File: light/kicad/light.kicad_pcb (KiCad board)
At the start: 4 copper layers, 24 x 55.9 mm, 103 parts, among them J1 Conn_01x03_Pin, J2 Conn_01x02_Pin, J3 SPI Socket, U1 FT4232H, U11 TLV7103318DDSE, U14 74LVC1G07, U2 SN74AVC4T774RSVR, U3 SN74AVC4T774RSVR, U4 SN74AVC4T774RSVR, U5 74LVC1G07, U6 SN74AHC595QWBQBRQ1, U7 TLV75533PDBV, U8 TLV75533PDBV, U9 93LC56BT-I/OT, Y1 12MHz_7M-12.000MAAJ

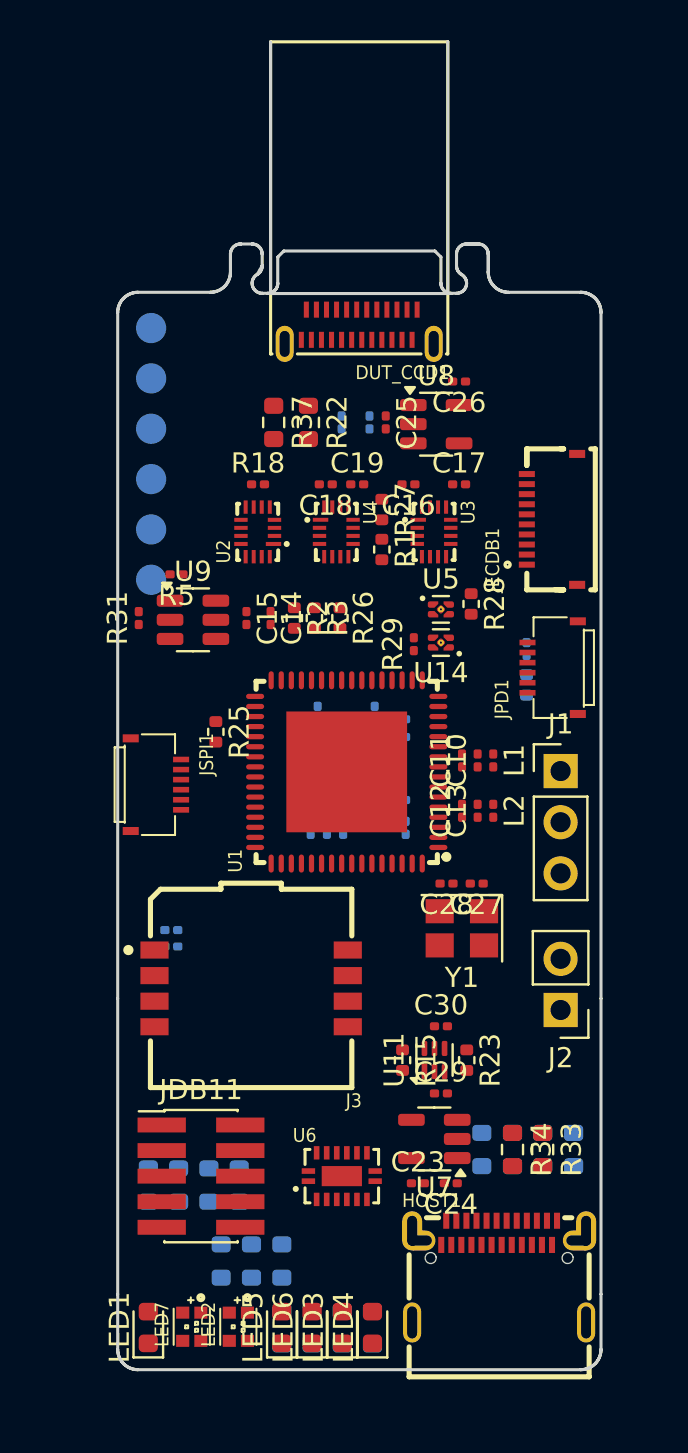
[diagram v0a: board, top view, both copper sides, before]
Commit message: kicad: Update board file layout routing
update board file.
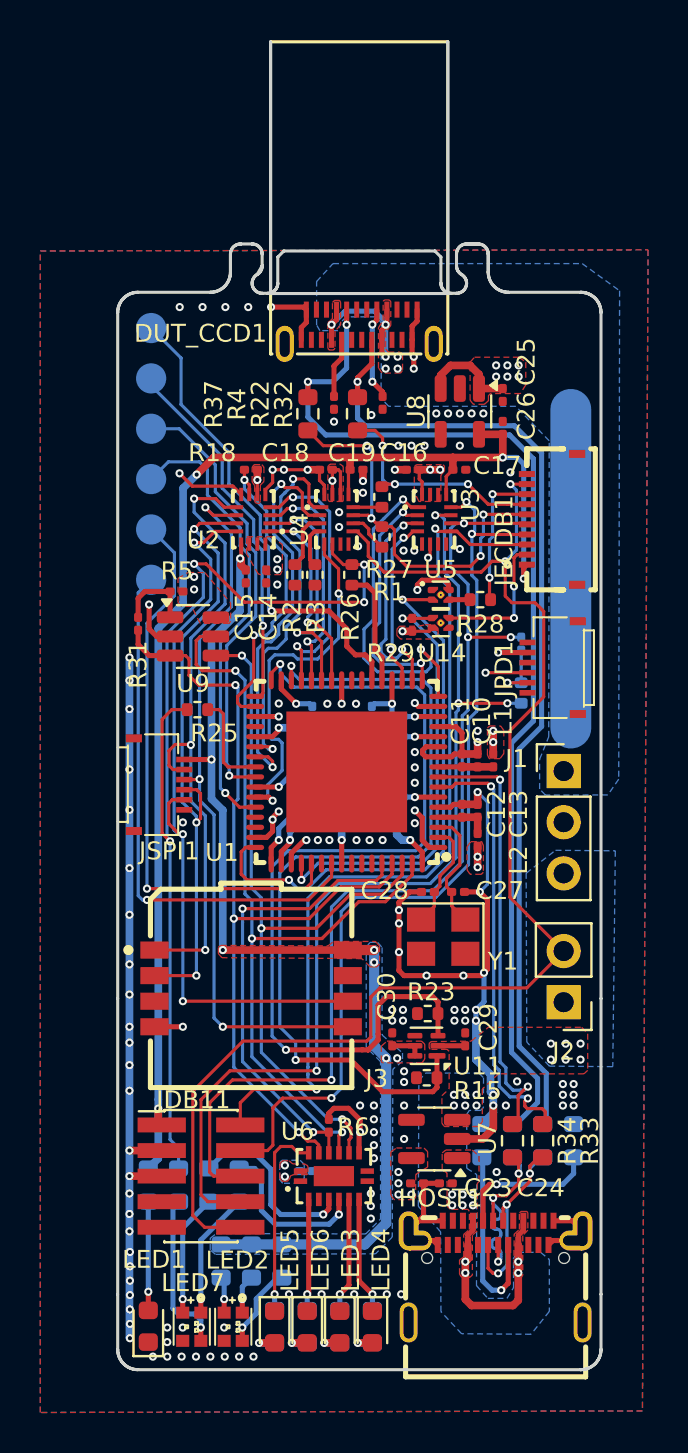
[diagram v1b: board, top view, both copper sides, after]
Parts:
- R32, R4, R6: moved to F.Cu
- moved C22 13.0 mm to (239.4, 119.7)
- moved R6 12.5 mm to (240.6, 117.4), turned to -90 degrees
- moved C25 5.97 mm to (249.2, 81.1)
- moved C26 3.16 mm to (249.2, 82.8), turned to 90 degrees
- moved R23 3.02 mm to (245.5, 111.9), turned to 0 degrees
- moved C29 2.94 mm to (247.4, 113.1), turned to 90 degrees
- moved C30 2.51 mm to (243.7, 113.1), turned to 90 degrees
- moved R22 2.48 mm to (242.0, 82.1)
- moved R26 2.23 mm to (241.7, 90.1)
- moved R2 2.15 mm to (238.9, 90.1)
- moved R3 2.15 mm to (239.9, 90.1)
- moved C14 2.08 mm to (237.5, 90.2)
- moved C15 2.07 mm to (236.5, 90.2)
- moved R37 1.75 mm to (239.5, 82.1)
- moved L2 1.64 mm to (248.0, 103.2), turned to 90 degrees
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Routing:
- net GND: track 0.00 -> 118.1 mm, vias 0 -> 142
- net /~{EC_RST}: track 0.00 -> 67.9 mm, vias 0 -> 2
- net EC_VREF: track 0.00 -> 65.7 mm, vias 0 -> 4
- net AP_SPI_VREF: track 0.00 -> 54.7 mm, vias 0 -> 7
- net /DUT_CCD_SBU2: track 0.00 -> 54.3 mm, vias 0 -> 2
- net /EC_RST_UNSHIFTED: track 0.00 -> 52.0 mm, vias 0 -> 4
- net /EC_JTAG_TDO: track 0.00 -> 51.8 mm, vias 0 -> 4
- net /EC_JTAG_TDI: track 0.00 -> 50.9 mm, vias 0 -> 4
- net /DUT_CCD_SBU1: track 0.00 -> 49.2 mm, vias 0 -> 1
- net /EC_JTAG_TCK: track 0.00 -> 45.6 mm, vias 0 -> 3
- net /SPI_VREF_FORCE_1.8: track 0.00 -> 45.3 mm, vias 0 -> 2
- net /EC_JTAG_TMS: track 0.00 -> 44.1 mm, vias 0 -> 2
- net /SPI_VREF_FORCE_3.3: track 0.00 -> 43.1 mm, vias 0 -> 2
- net /EEDATA: track 0.00 -> 41.5 mm, vias 0 -> 3
- net /EECS: track 0.00 -> 40.9 mm, vias 0 -> 3
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- added copper zone on B.Cu, net 3.3V
- added copper zone on F.Cu, net 3.3V
- added copper zone on In2.Cu, net 3.3V
- added copper zone on B.Cu, net AP_SPI_VREF
- added copper zone on F.Cu, net AP_SPI_VREF
- added copper zone on B.Cu, net CCD_VBUS
- added copper zone on F.Cu, net CCD_VBUS
- added copper zone on In2.Cu, net CCD_VBUS
- added copper zone on B.Cu, net GND
- added copper zone on F.Cu, net GND
- added copper zone on In1.Cu, net GND
- added copper zone on B.Cu, net HOST_VBUS
- added copper zone on F.Cu, net HOST_VBUS
- added copper zone on In2.Cu, net HOST_VBUS
- added copper zone on F.Cu, net Net-(J1-Pin_2)
- added copper zone on In1.Cu, net Net-(J1-Pin_2)
